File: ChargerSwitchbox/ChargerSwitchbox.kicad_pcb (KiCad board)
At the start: 2 copper layers, 71.8 x 48.3 mm, 16 parts, among them J1 Charger Control, J2 Charger LV, J3 Charger Current Direct, J4 Estop Connector, J5 Charger Current Out, J6 Connector Interlock, U1 G2RL-1A-E, U2 G2RL-1A-E, U3 G2RL-1A-E

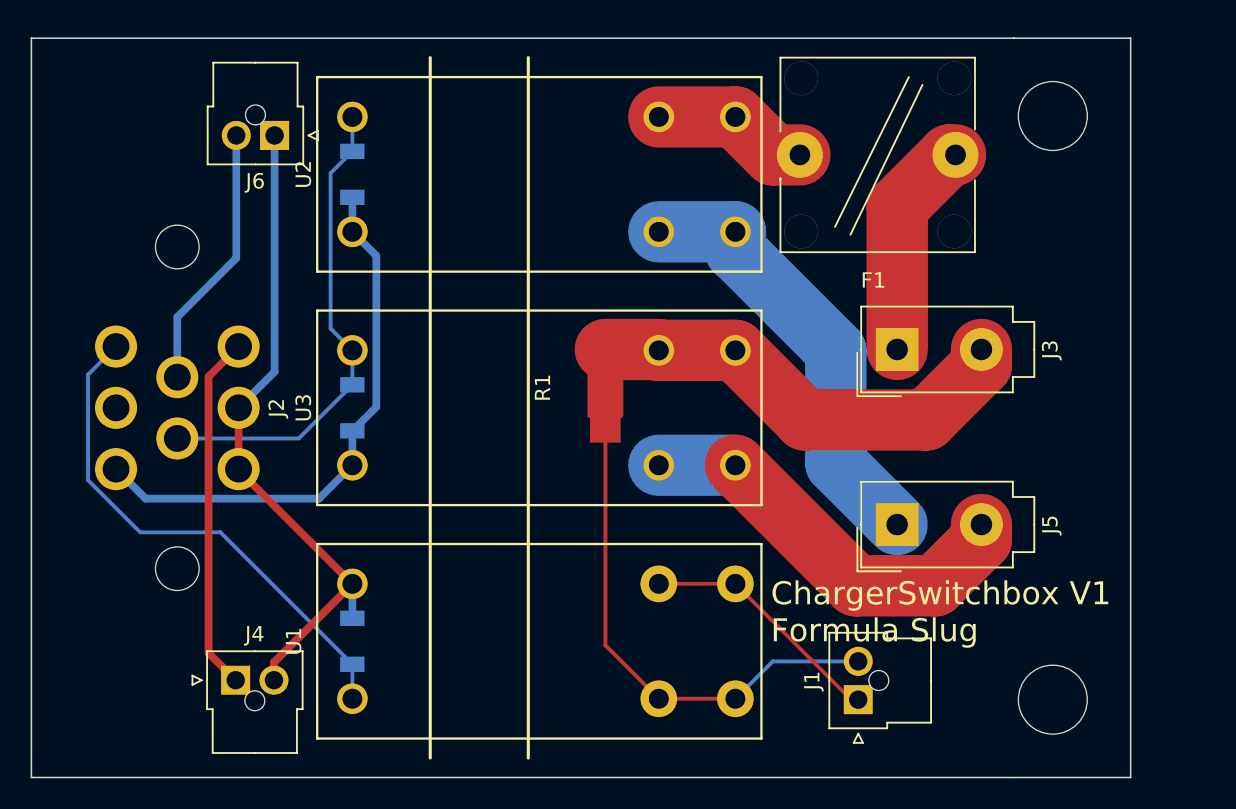
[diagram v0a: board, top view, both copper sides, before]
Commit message: hopefully finalize PCBs for send to manufacturing
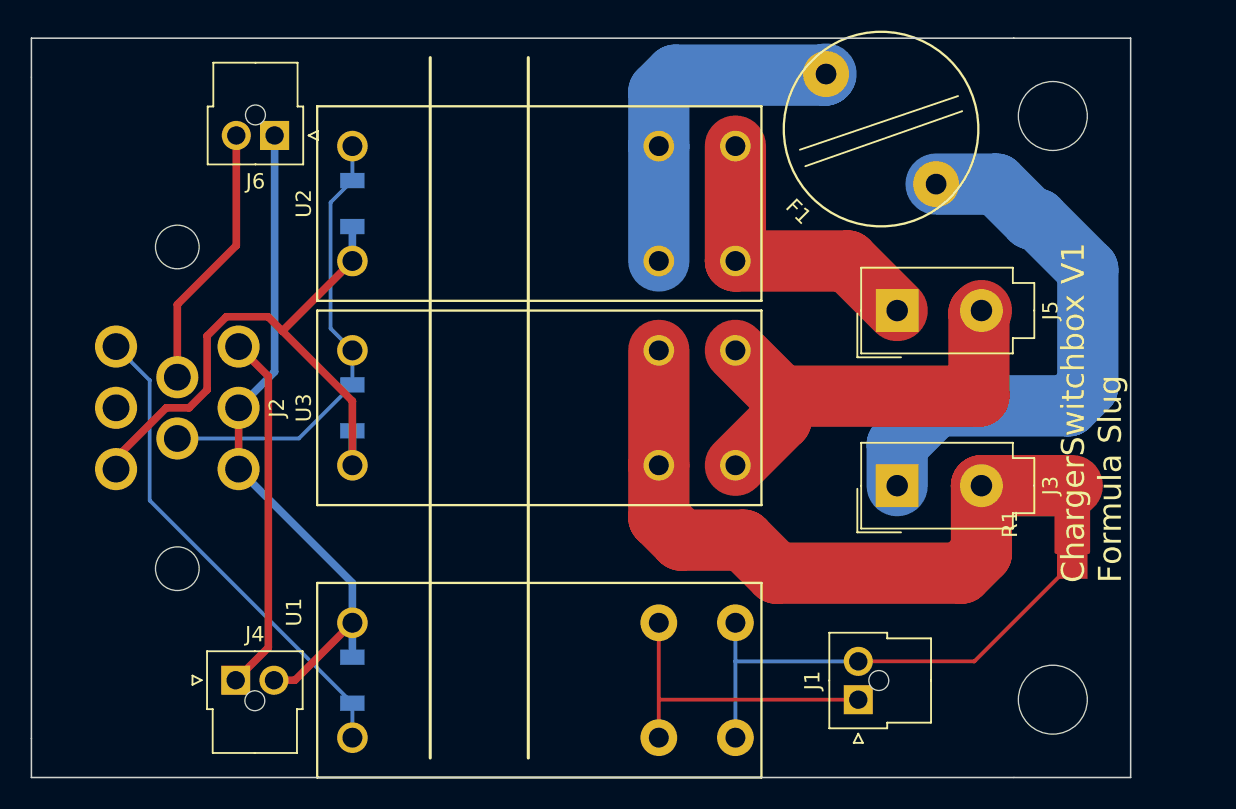
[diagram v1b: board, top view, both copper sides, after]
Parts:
- F1: footprint Fuse_Holders_and_Fuses:Fuseholder5x20_vert_closed_Bulgin_FX0456 -> FSFootprints:Fuseholder5x20_vert
- moved R1 31.7 mm to (200.7, 57.1)
- moved J5 14.0 mm to (189.2, 43.2)
- moved J3 8.89 mm to (189.2, 54.6)
- moved D1 2.54 mm to (153.7, 67.3)
- moved U1 2.54 mm to (153.7, 67.3)
- moved F1 2.29 mm to (191.8, 34.9), turned to 135 degrees
- moved D2 1.91 mm to (153.7, 36.2)
- moved U2 1.91 mm to (153.7, 36.2)
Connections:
- U1 pad 4: /CHARGER_TEMP -> Net-(J1-Pad2)
- U1 pad 6: Net-(J1-Pad2) -> /CHARGER_TEMP
- U2 pad 4: /CHARGER_OUT+_FUSED -> /CHARGER+
- U2 pad 6: /CHARGER+ -> /CHARGER_OUT+_FUSED
- U3 pad 4: /CHARGER_OUT- -> /CHARGER-
- U3 pad 6: /CHARGER- -> /CHARGER_OUT-
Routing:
- net /CHARGER_OUT+: track 14.5 -> 36.5 mm
- net /CHARGER_OUT-: track 29.0 -> 44.4 mm
- net /CHARGER_OUT+_FUSED: track 10.2 -> 22.5 mm
- net /CHARGER+: track 28.5 -> 19.4 mm
- net /CHARGER_TEMP: track 16.2 -> 20.5 mm
- net GND: track 35.9 -> 39.5 mm
- net /CHARGER_CONTROL: track 34.0 -> 31.9 mm
- net /CHARGER-: track 26.5 -> 28.5 mm
- net /AIRS_FINAL_CHARGER: track 31.6 -> 29.6 mm
- net Net-(J1-Pad2): track 33.2 -> 32.1 mm
- net +12V: track 44.0 -> 44.8 mm
